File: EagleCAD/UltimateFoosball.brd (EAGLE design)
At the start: 87 x 93 mm, 28 parts

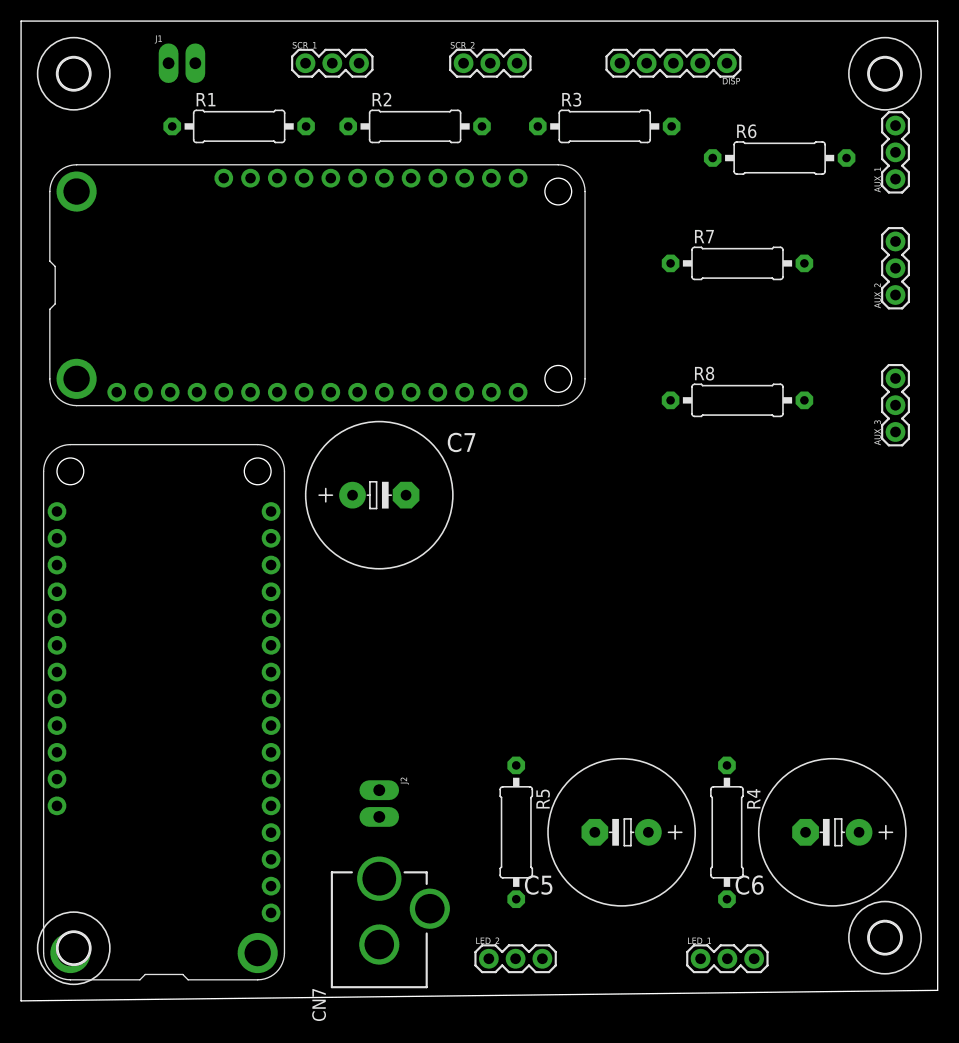
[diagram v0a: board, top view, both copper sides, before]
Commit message: Version 1 complete, sent to OSHPark
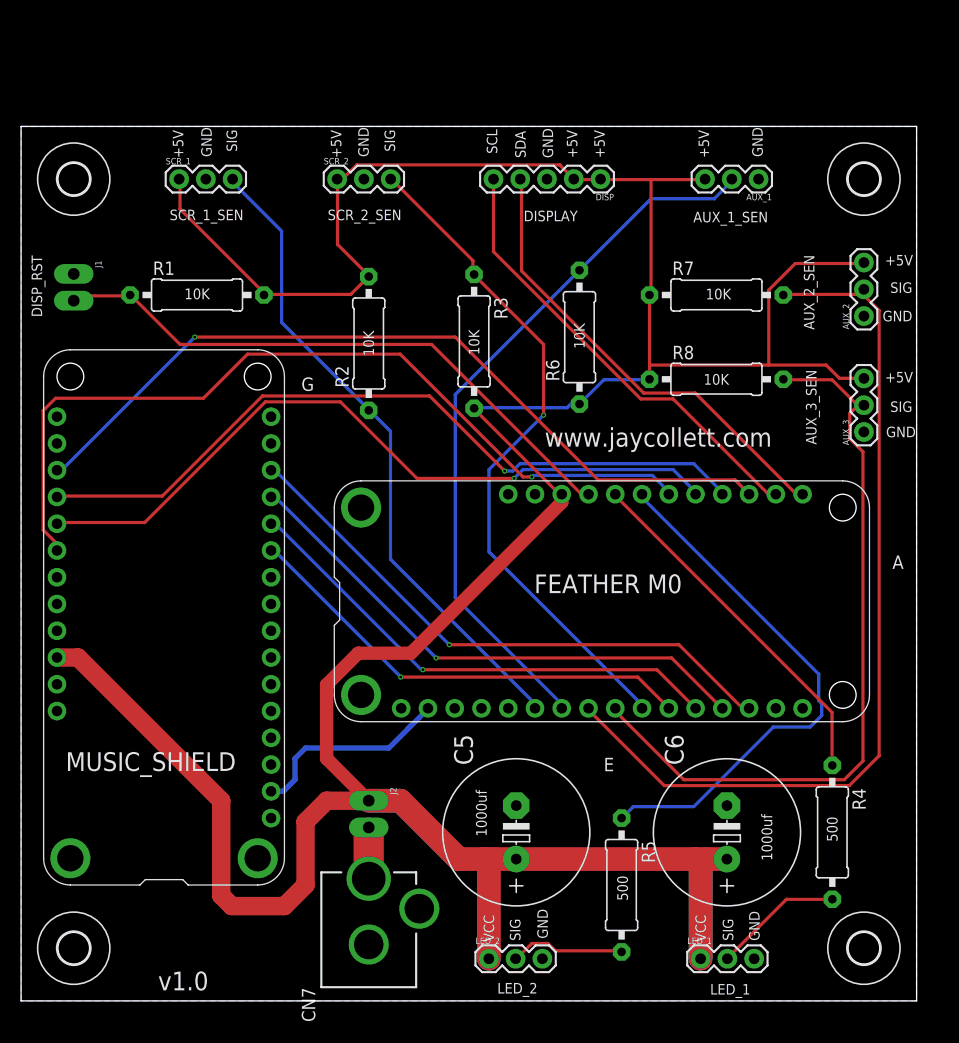
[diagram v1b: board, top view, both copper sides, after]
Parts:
- removed C7: (no value), adafruit:E5-13
- moved MS1 40.4 mm to (29.7, 26.5)
- moved R6 25.5 mm to (53.0, 63.0), turned to 90 degrees
- moved R3 23.9 mm to (43.0, 62.6), turned to 270 degrees
- moved J1 21.9 mm to (5.00, 69.0), turned to 270 degrees
- moved R2 21.1 mm to (33.0, 62.4), turned to 90 degrees
- moved R1 16.5 mm to (16.7, 67.0)
- moved DISP 16.3 mm to (55.0, 78.0)
- moved SCR_1 16.3 mm to (15.0, 78.0)
- moved SCR_2 16.3 mm to (30.0, 78.0)
- moved AUX_1 13.0 mm to (70.0, 78.0), turned to 180 degrees
- moved R5 11.2 mm to (57.0, 11.0)
- moved H2 10.2 mm to (80.0, 78.0)
- moved C5 10.0 mm to (47.0, 16.0), turned to 90 degrees
- moved C6 10.0 mm to (67.0, 16.0), turned to 90 degrees
- moved H1 10.0 mm to (5.00, 78.0)
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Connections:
- net +5V: no longer C7.+
- net GND: no longer C7.-
- net RST_DISP: now also MS1.25
- net SCR_1_SIG: now also MS1.6
- net SCR_2_SIG: now also MS1.10
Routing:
- net +5V: track 0.00 -> 364.8 mm
- net AUX_2_SIG: track 0.00 -> 84.8 mm
- net XDCS: track 0.00 -> 81.3 mm, vias 0 -> 1
- net SD_CS: track 0.00 -> 77.1 mm, vias 0 -> 1
- net MP3CS: track 0.00 -> 71.7 mm, vias 0 -> 1
- net AUX_3_SIG: track 0.00 -> 71.0 mm
- net DREQ: track 0.00 -> 69.9 mm, vias 0 -> 1
- net AUX_1_SIG: track 0.00 -> 68.9 mm
- net SCR_2_SIG: track 0.00 -> 64.5 mm, vias 0 -> 1
- net SCR_1_SIG: track 0.00 -> 62.1 mm
- net RST_DISP: track 0.00 -> 57.0 mm
- net MIDI: track 0.00 -> 54.8 mm, vias 0 -> 1
- net GPIOMISO: track 0.00 -> 51.1 mm, vias 0 -> 1
- net LED_SIG_2: track 0.00 -> 51.1 mm
- net GPIOMOSI: track 0.00 -> 47.5 mm, vias 0 -> 1
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- added copper zone on layer 16, net GND
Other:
- board size 87 x 93 mm -> 85 x 83 mm
- board text added: "+5V"
- board text added: "1000uf"
- board text added: "10K"
- board text added: "500"
- board text added: "A"
- board text added: "AUX_1_SEN"
- board text added: "AUX_2_SEN"
- board text added: "AUX_3_SEN"
- board text added: "Always be curious my kids..."
- board text added: "DISPLAY"
- board text added: "DISP_RST"
- board text added: "E"
- board text added: "FEATHER M0"
- board text added: "G"
- board text added: "GND"
- board text added: "LED_1"
- board text added: "LED_2"
- board text added: "MUSIC_SHIELD"
- board text added: "SCL"
- board text added: "SCR_1_SEN"
- board text added: "SCR_2_SEN"
- board text added: "SDA"
- board text added: "SIG"
- board text added: "VCC"
- board text added: "v1.0"
- board text added: "www.jaycollett.com"
